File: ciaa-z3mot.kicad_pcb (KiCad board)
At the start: 2 copper layers, 18.8 x 67.7 mm, 78 parts, among them J1 Conn_01x20, J2 Conn_01x20, J3 Conn_01x02, J4 SWD, J5 Conn_01x04, J6 Conn_Coaxial, J7 Conn_01x05, J8 Conn_Coaxial, SW1 reset, SW2 reset, U1 EZM32HG320-48QFP, U2 24AA02E48-OT, U3 USBLC6-2, U4 SPX3819M5-L-3-3, U5 USB_PCB_PRINT, U6 MCP1640BCH, Y1 30MHz, Y2 32.1KHz, Y3 24MHz

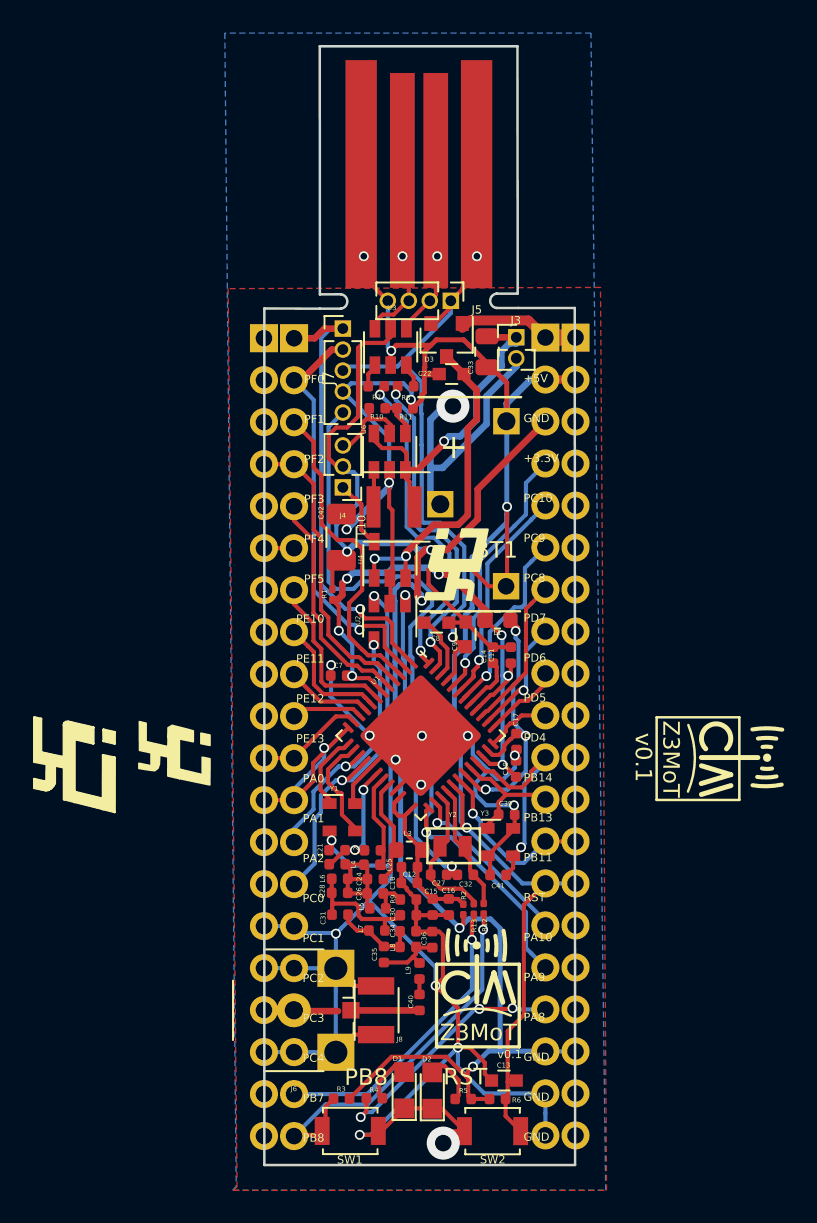
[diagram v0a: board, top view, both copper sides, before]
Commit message: more readme!!! ):
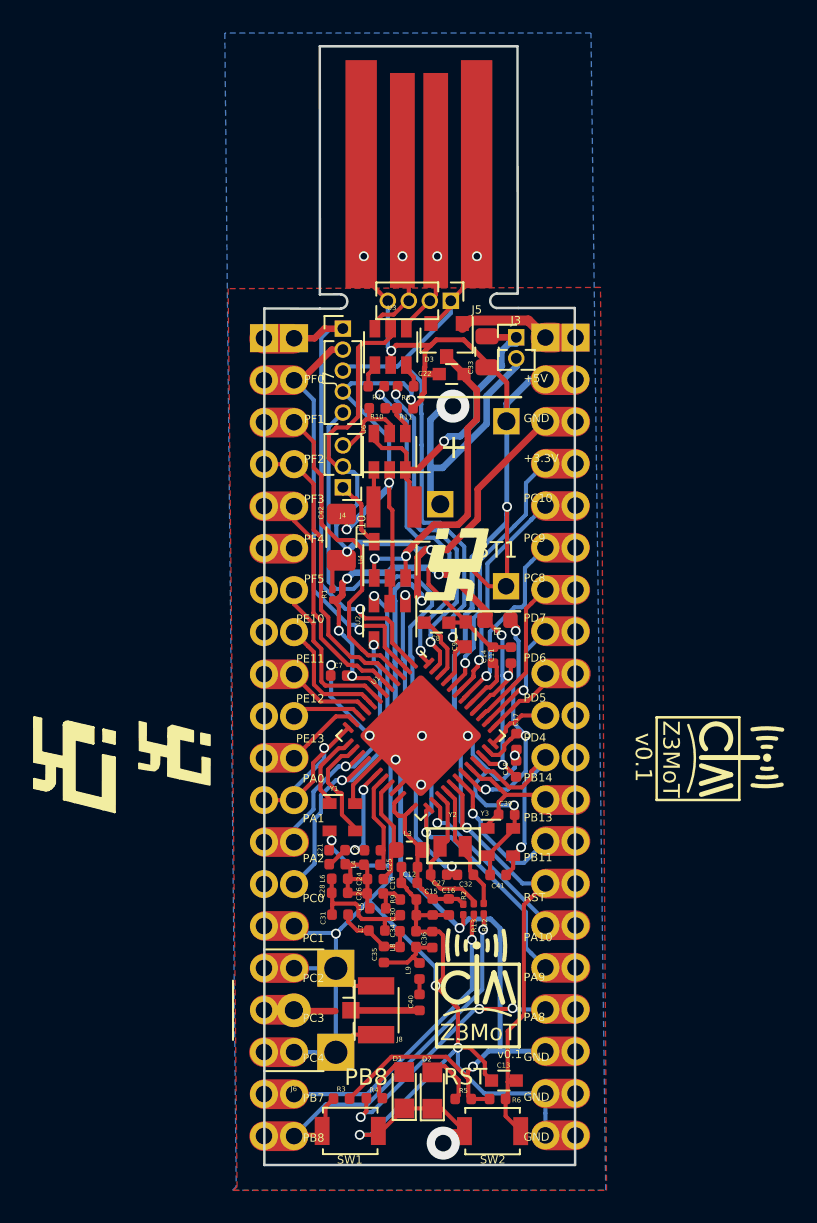
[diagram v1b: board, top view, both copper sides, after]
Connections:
- BT1 pad 3: (no net) -> GND
- U1 pad : (no net) -> GND
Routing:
- net GND: track 239.3 -> 251.7 mm
- net +3V3: track 95.5 -> 99.0 mm
- net /PC10: track 15.8 -> 17.6 mm
- net HFXTAL_P: track 7.78 -> 9.55 mm
- net /nRESET: track 61.2 -> 63.0 mm
- net /PF5: track 1.40 -> 3.17 mm
- net /PF4: track 14.0 -> 15.8 mm
- net /PF2: track 19.7 -> 21.4 mm
- net /PF1/SWDIO: track 25.9 -> 27.7 mm
- net /PF0/SWCLK: track 28.0 -> 29.8 mm
- net /PE12: track 5.41 -> 7.18 mm
- net /PD7: track 9.30 -> 11.1 mm
- net /PD6: track 7.07 -> 8.84 mm
- net /PD5: track 4.88 -> 6.65 mm
- net /PC9: track 13.6 -> 15.3 mm
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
